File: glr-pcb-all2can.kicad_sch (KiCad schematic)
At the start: 19 parts, among them J1 Conn_02x04_Top_Bottom, J2 DA15_Pins_MountingHoles, U1 STM32F303K8T6, U2 173020536, U3 173010535

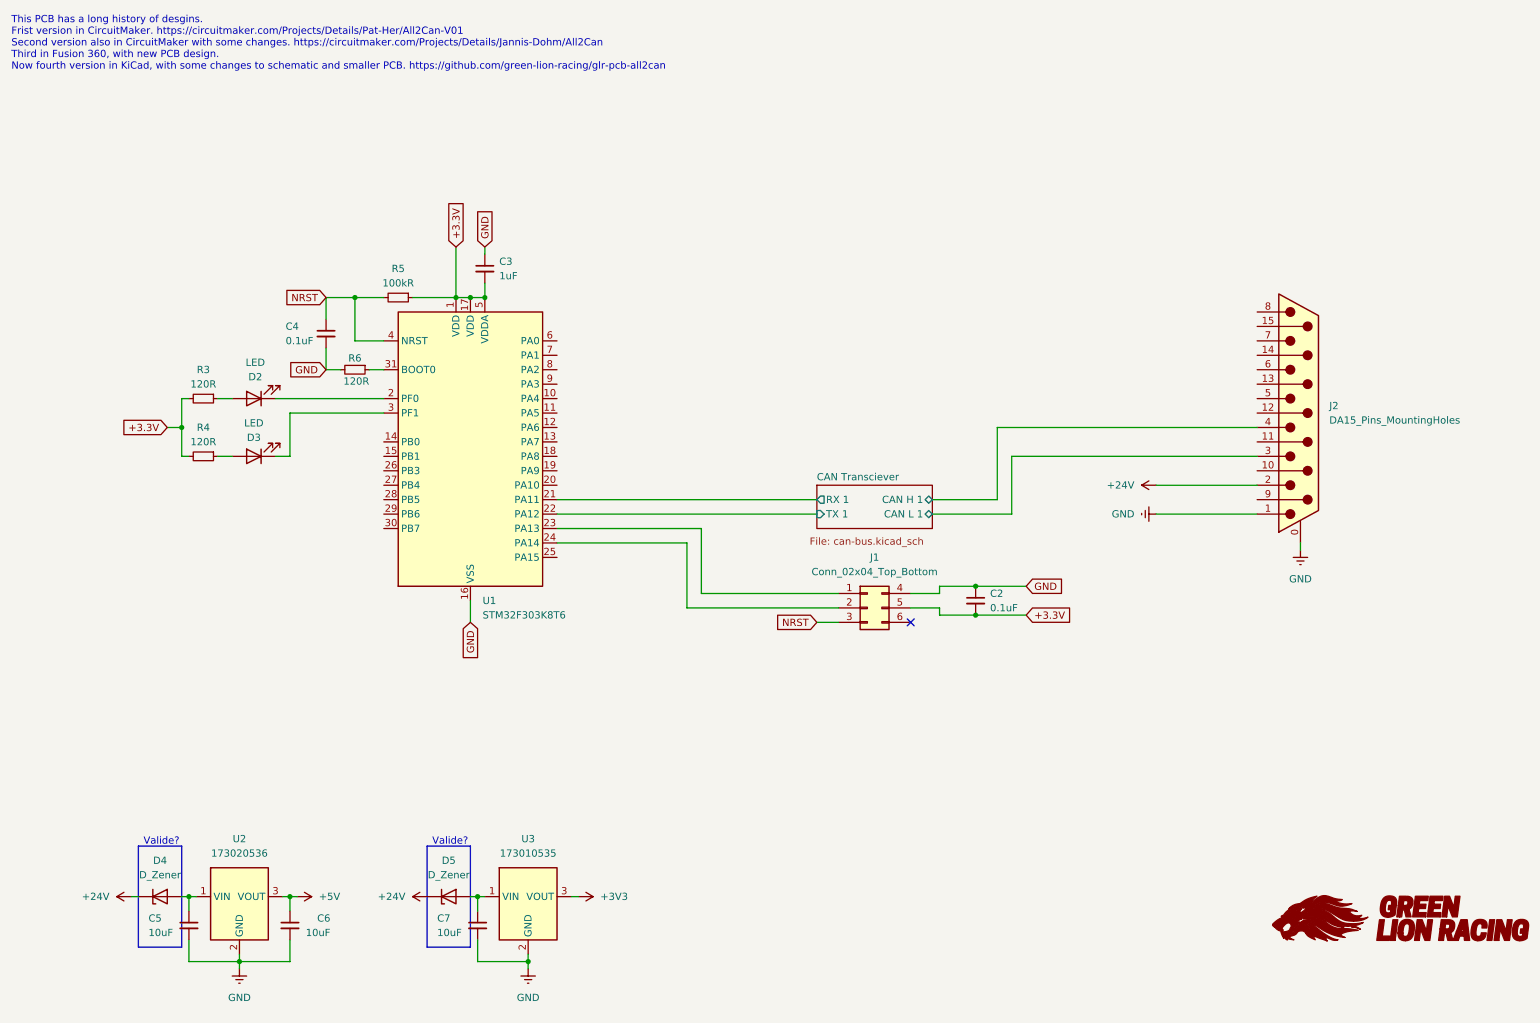
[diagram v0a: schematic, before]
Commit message: add in- and outputs
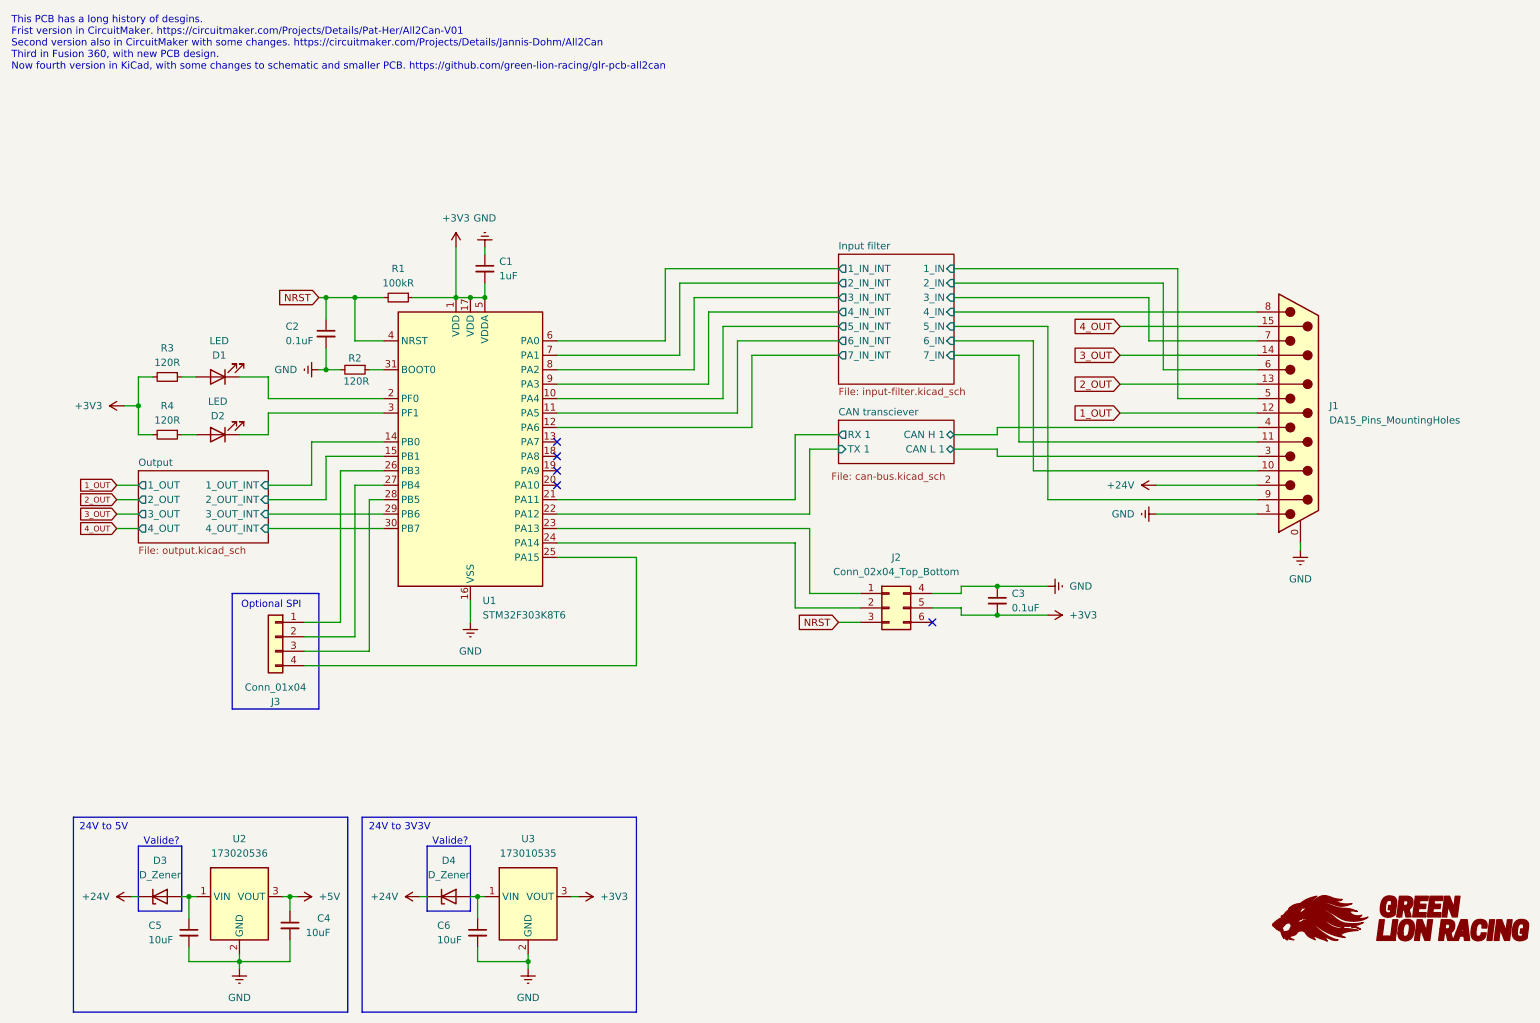
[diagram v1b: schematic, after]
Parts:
- added J3: Conn_01x04, Connector_PinSocket_2.54mm:PinSocket_1x04_P2.54mm_Vertical, symbol Connector_Generic:Conn_01x04
- renumbered C3 to C1, C4 to C2, C2 to C3, C6 to C4, C7 to C6, D2 to D1, D3 to D2, D4 to D3, D5 to D4, J2 to J1, J1 to J2, R5 to R1, R6 to R2
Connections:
- net +3.3V is gone; now on net +3V3: C1.2, C3.2, J2.5 (Pin_5), R1.1, R3.2, R4.2, U1.1 (VDD), U1.17 (VDD), U1.5 (VDDA)
- net Input filter/5_IN_INT: now reaches U1.10 (PA4)
- net Input filter/6_IN_INT: now reaches U1.11 (PA5)
- net Input filter/7_IN_INT: now reaches U1.12 (PA6)
- net Output/1_OUT_INT: now reaches U1.14 (PB0)
- net Output/2_OUT_INT: now reaches U1.15 (PB1)
- net at U1.25 (PA15): now also J3.4 (Pin_4)
- net at U1.26 (PB3): now also J3.1 (Pin_1)
- net at U1.27 (PB4): now also J3.2 (Pin_2)
- net at U1.28 (PB5): now also J3.3 (Pin_3)
- net Output/3_OUT_INT: now reaches U1.29 (PB6)
- net Output/4_OUT_INT: now reaches U1.30 (PB7)
- net Input filter/1_IN_INT: now reaches U1.6 (PA0)
- net Input filter/2_IN_INT: now reaches U1.7 (PA1)
- net Input filter/3_IN_INT: now reaches U1.8 (PA2)
- net Input filter/4_IN_INT: now reaches U1.9 (PA3)
- net Input filter/6_IN: now reaches J1.10 (P10)
- net Input filter/7_IN: now reaches J1.11 (P111)
- net 1_OUT: now reaches J1.12 (P12)
- net 2_OUT: now reaches J1.13 (P13)
- net 3_OUT: now reaches J1.14 (P14)
- net 4_OUT: now reaches J1.15 (P15)
- net Input filter/1_IN: now reaches J1.5
- net Input filter/2_IN: now reaches J1.6
- net Input filter/3_IN: now reaches J1.7
- net Input filter/4_IN: now reaches J1.8
- net Input filter/5_IN: now reaches J1.9 (P9)
- no-connect marks 1 -> 5
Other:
- sheet CAN Transciever renamed CAN transciever
- added sheet Input filter (input-filter.kicad_sch)
- added sheet Output (output.kicad_sch)
- note added: "24V to 3V3V"
- note added: "24V to 5V"
- note added: "Optional SPI"
- moved on the sheet: C3, C5, C6, D1, D2, J2, R3, R4
